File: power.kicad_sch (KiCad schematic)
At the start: 74 parts, among them Q1 BC817, Q2 BC817, Q3 BC817, Q4 AO3401A, U1 MP1470, U2 MP1470, U3 MP1470, U4 MP1470

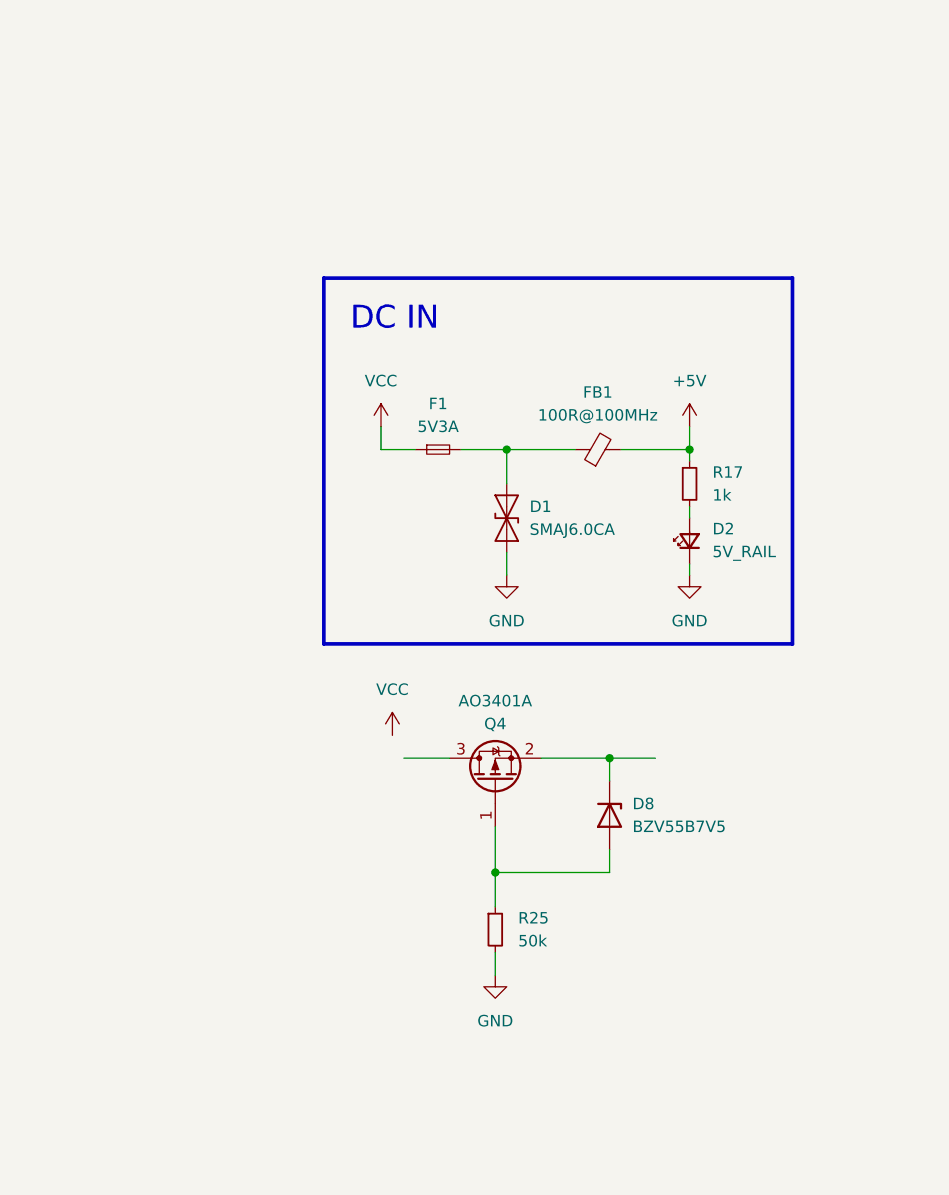
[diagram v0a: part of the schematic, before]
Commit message: first prototype. power sheet done
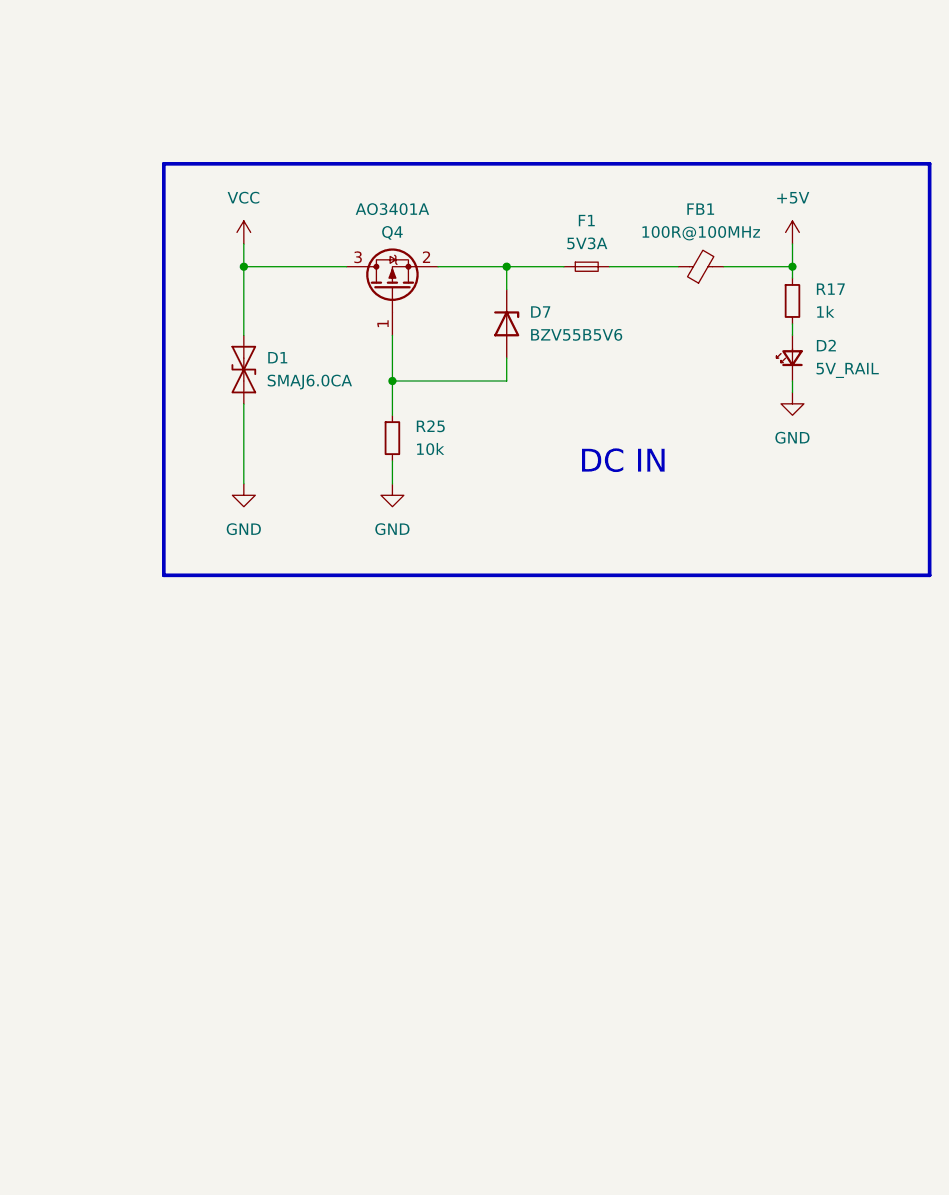
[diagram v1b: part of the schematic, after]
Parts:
- removed D8: BZV55B7V5, Diode_SMD:D_MiniMELF, symbol Diode:BZV55B7V5
- added D7: BZV55B5V6, Diode_SMD:D_MiniMELF, symbol Diode:BZV55B5V6
- R25: value 50k -> 10k
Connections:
- net VCC: now also D1.2 (A2), Q4.3 (D); no longer F1.1
- net at F1.2, FB1.1: no longer D1.2 (A2)
- net at Q4.2 (S): now also F1.1, D7.1 (K)
- net at Q4.1 (G), R25.1: now also D7.2 (A)
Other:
- moved on the sheet: D2, F1, FB1, Q4, R17, R25
